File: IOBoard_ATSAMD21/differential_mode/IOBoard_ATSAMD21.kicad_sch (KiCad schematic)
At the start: 74 parts, among them IC1 AD8137YRZ-REEL, IC2 AD8137YRZ-REEL, J13 Eurorack_Mono_Jack, J3 Conn_PIC_ICSP_ICD, J5 Conn_01x05_Pin, J6 Conn_02x03_Odd_Even, SW1 EG_1218, SW2 EG_1218, SW3 EG_1218, SW4 EG_1218, U3 ATSAMD21G18A-A, U4 LM2904, U6 AP2112K-3.3

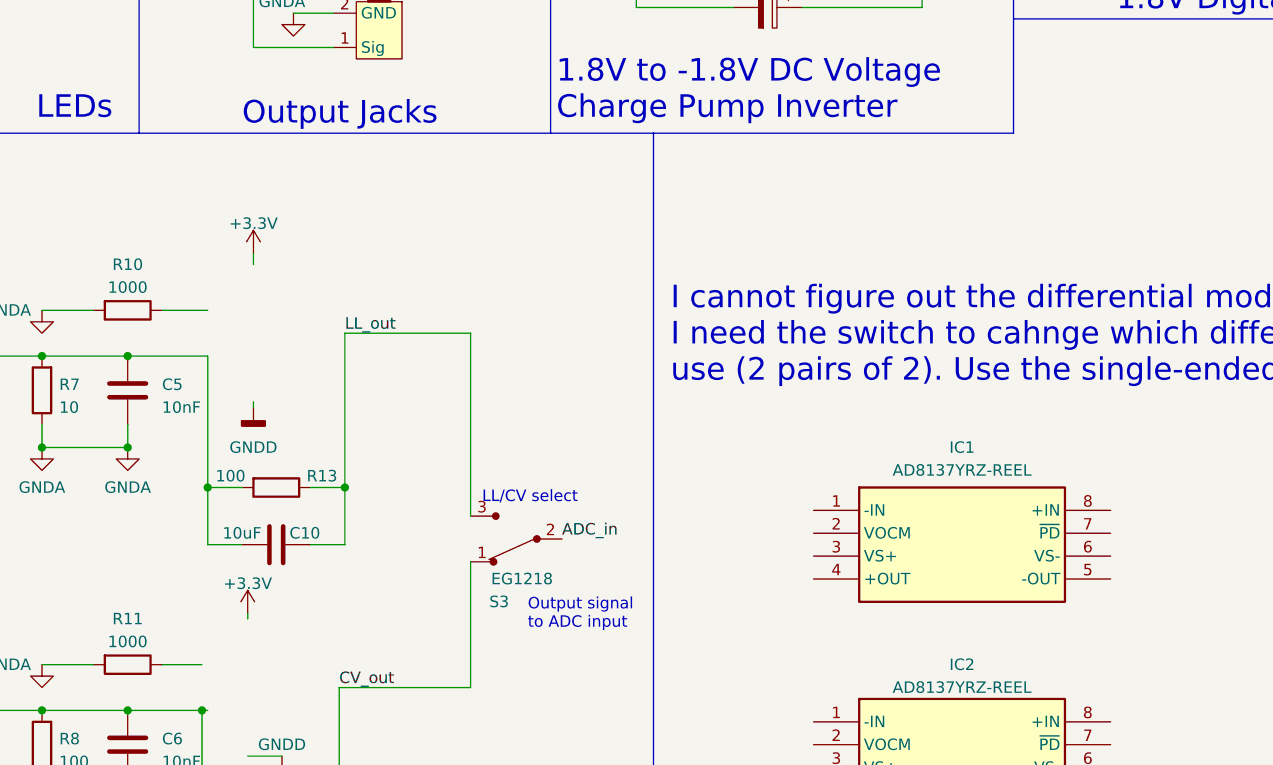
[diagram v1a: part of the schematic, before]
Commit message: plz work
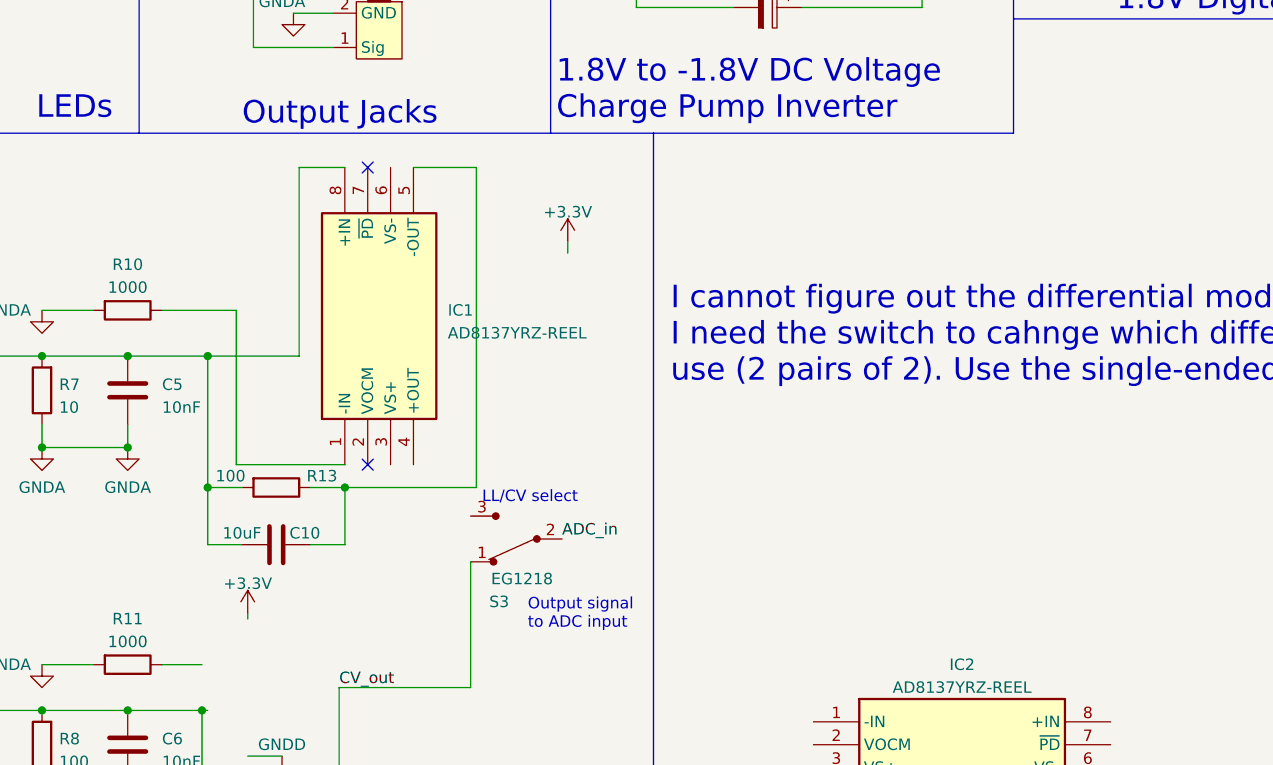
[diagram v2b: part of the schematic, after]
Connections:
- net LL_out: no longer C10.1, R13.1, S3.3
- net at C10.2, C5.2, R13.2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: now also IC1.8 (+IN)
- net at IC1.1 (-IN): now also R10.1
- net at IC1.5 (-OUT): now also C10.1, R13.1
- no-connect marks 7 -> 9
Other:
- moved on the sheet: IC1
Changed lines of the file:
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@@
   (junction (at 50.165 187.325) (diameter 0) (color 0 0 0 0)
   )
+  (junction (at 127 238.125) (diameter 0) (color 0 0 0 0)
+  )
   (junction (at 111.125 272.415) (diameter 0) (color 0 0 0 0)
   )
@@
   (junction (at 111.76 137.795) (diameter 0) (color 0 0 0 0)
   )
-  (junction (at 127 238.125) (diameter 0) (color 0 0 0 0)
-  )
   (junction (at 93.345 223.52) (diameter 0) (color 0 0 0 0)
   )
@@
   (junction (at 256.54 123.825) (diameter 0) (color 0 0 0 0)
   )
+  (junction (at 111.76 223.52) (diameter 0) (color 0 0 0 0)
+  )
   (junction (at 102.87 280.67) (diameter 0) (color 0 0 0 0)
   )
@@
   (no_connect (at 187.325 172.085))
   (no_connect (at 125.73 171.45))
+  (no_connect (at 129.54 202.565))
+  (no_connect (at 129.54 235.585))
   (no_connect (at 235.585 147.955))
   (no_connect (at 220.345 150.495))
@@
     (stroke (width 0) (type default))
   )
+  (wire (pts (xy 114.935 235.585) (xy 114.935 218.44))
+    (stroke (width 0) (type default))
+  )
   (wire (pts (xy 126.365 281.305) (xy 126.365 276.225))
     (stroke (width 0) (type default))
@@
     (stroke (width 0) (type default))
   )
+  (wire (pts (xy 121.92 202.565) (xy 121.92 223.52))
+    (stroke (width 0) (type default))
+  )
   (wire (pts (xy 114.3 64.135) (xy 121.92 64.135))
     (stroke (width 0) (type default))
@@
     (stroke (width 0) (type default))
   )
-  (wire (pts (xy 106.68 218.44) (xy 111.76 218.44))
+  (wire (pts (xy 106.68 218.44) (xy 114.935 218.44))
     (stroke (width 0) (type default))
   )
@@
     (stroke (width 0) (type default))
   )
-  (wire (pts (xy 140.97 241.3) (xy 140.97 220.98))
-    (stroke (width 0) (type default))
-  )
   (wire (pts (xy 137.16 20.955) (xy 137.16 26.035))
     (stroke (width 0) (type default))
@@
     (stroke (width 0) (type default))
   )
-  (wire (pts (xy 140.97 220.98) (xy 127 220.98))
-    (stroke (width 0) (type default))
-  )
   (polyline (pts (xy 201.295 198.755) (xy 201.295 159.385))
     (stroke (width 0) (type default))
@@
     (stroke (width 0) (type default))
   )
+  (wire (pts (xy 121.92 223.52) (xy 111.76 223.52))
+    (stroke (width 0) (type default))
+  )
   (wire (pts (xy 137.16 31.115) (xy 140.97 31.115))
     (stroke (width 0) (type default))
@@
     (stroke (width 0) (type default))
   )
-  (wire (pts (xy 116.84 229.235) (xy 116.84 228.6))
-    (stroke (width 0) (type default))
-  )
   (wire (pts (xy 266.7 34.925) (xy 271.78 34.925))
     (stroke (width 0) (type default))
@@
     (stroke (width 0) (type default))
   )
+  (wire (pts (xy 141.605 202.565) (xy 141.605 238.125))
+    (stroke (width 0) (type default))
+  )
   (wire (pts (xy 40.64 36.195) (xy 40.64 40.005))
     (stroke (width 0) (type default))
@@
     (stroke (width 0) (type default))
   )
-  (wire (pts (xy 116.84 212.09) (xy 116.84 213.36))
+  (wire (pts (xy 151.765 210.82) (xy 151.765 212.09))
     (stroke (width 0) (type default))
   )
@@
     (stroke (width 0) (type default))
   )
-  (wire (pts (xy 127 220.98) (xy 127 238.125))
-    (stroke (width 0) (type default))
-  )
   (wire (pts (xy 39.37 95.885) (xy 41.91 95.885))
     (stroke (width 0) (type default))
@@
     (stroke (width 0) (type default))
   )
+  (wire (pts (xy 134.62 202.565) (xy 141.605 202.565))
+    (stroke (width 0) (type default))
+  )
   (wire (pts (xy 114.3 64.135) (xy 114.3 69.215))
     (stroke (width 0) (type default))
@@
     (stroke (width 0) (type default))
   )
+  (wire (pts (xy 127 202.565) (xy 121.92 202.565))
+    (stroke (width 0) (type default))
+  )
   (polyline (pts (xy 215.9 104.775) (xy 215.9 127.635))
     (stroke (width 0) (type default))
@@
     (stroke (width 0) (type default))
   )
+  (wire (pts (xy 141.605 238.125) (xy 127 238.125))
+    (stroke (width 0) (type default))
+  )
   (wire (pts (xy 223.52 64.135) (xy 226.06 64.135))
     (stroke (width 0) (type default))
@@
     (stroke (width 0) (type default))
   )
+  (wire (pts (xy 127 235.585) (xy 114.935 235.585))
+    (stroke (width 0) (type default))
+  )
   (wire (pts (xy 241.3 64.135) (xy 241.3 53.975))
     (stroke (width 0) (type default))
@@
     (effects (font (size 1.27 1.27)) (justify left bottom))
   )
-  (label "LL_out" (at 127 220.98 0) (fields_autoplaced)
-    (effects (font (size 1.27 1.27)) (justify left bottom))
-  )
   (label "LED3" (at 72.39 164.465 90) (fields_autoplaced)
     (effects (font (size 1.27 1.27)) (justify left bottom))
@@
     )
   )
-  (symbol (lib_id "AD8137YRZ-REEL:AD8137YRZ-REEL") (at 179.07 240.665 0) (unit 1)
-    (in_bom yes) (on_board yes) (dnp no) (fields_autoplaced)
-    (property "Reference" "IC1" (at 195.58 233.68 0)
-      (effects (font (size 1.27 1.27)))
+  (symbol (lib_id "AD8137YRZ-REEL:AD8137YRZ-REEL") (at 127 235.585 90) (unit 1)
+    (in_bom yes) (on_board yes) (dnp no)
+    (property "Reference" "IC1" (at 138.43 218.44 90)
+      (effects (font (size 1.27 1.27)) (justify right))
     )
-    (property "Value" "AD8137YRZ-REEL" (at 195.58 236.22 0)
-      (effects (font (size 1.27 1.27)))
+    (property "Value" "AD8137YRZ-REEL" (at 138.43 220.98 90)
+      (effects (font (size 1.27 1.27)) (justify right))
     )
-    (property "Footprint" "SOIC127P600X175-8N" (at 208.28 335.585 0)
+    (property "Footprint" "SOIC127P600X175-8N" (at 221.92 206.375 0)
       (effects (font (size 1.27 1.27)) (justify left top) hide)
     )
-    (property "Datasheet" "https://www.arrow.com/en/products/ad8137yrz-reel/analog-devices" (at 208.28 435.585 0)
+    (property "Datasheet" "https://www.arrow.com/en/products/ad8137yrz-reel/analog-devices" (at 321.92 206.375 0)
       (effects (font (size 1.27 1.27)) (justify left top) hide)
     )
-    (property "Height" "1.75" (at 208.28 635.585 0)
+    (property "Height" "1.75" (at 521.92 206.375 0)
       (effects (font (size 1.27 1.27)) (justify left top) hide)
     )
-    (property "Manufacturer_Name" "Analog Devices" (at 208.28 735.585 0)
+    (property "Manufacturer_Name" "Analog Devices" (at 621.92 206.375 0)
       (effects (font (size 1.27 1.27)) (justify left top) hide)
     )
-    (property "Manufacturer_Part_Number" "AD8137YRZ-REEL" (at 208.28 835.585 0)
+    (property "Manufacturer_Part_Number" "AD8137YRZ-REEL" (at 721.92 206.375 0)
       (effects (font (size 1.27 1.27)) (justify left top) hide)
     )
-    (property "Mouser Part Number" "584-AD8137YRZ-R" (at 208.28 935.585 0)
+    (property "Mouser Part Number" "584-AD8137YRZ-R" (at 821.92 206.375 0)
       (effects (font (size 1.27 1.27)) (justify left top) hide)
     )
-    (property "Mouser Price/Stock" "https://www.mouser.co.uk/ProductDetail/Analog-Devices/AD8137YRZ-REEL?qs=%2FtpEQrCGXCwvx9BEhEk72g%3D%3D" (at 208.28 1035.585 0)
+    (property "Mouser Price/Stock" "https://www.mouser.co.uk/ProductDetail/Analog-Devices/AD8137YRZ-REEL?qs=%2FtpEQrCGXCwvx9BEhEk72g%3D%3D" (at 921.92 206.375 0)
       (effects (font (size 1.27 1.27)) (justify left top) hide)
     )
-    (property "Arrow Part Number" "AD8137YRZ-REEL" (at 208.28 1135.585 0)
+    (property "Arrow Part Number" "AD8137YRZ-REEL" (at 1021.92 206.375 0)
       (effects (font (size 1.27 1.27)) (justify left top) hide)
     )
-    (property "Arrow Price/Stock" "https://www.arrow.com/en/products/ad8137yrz-reel/analog-devices?region=nac" (at 208.28 1235.585 0)
+    (property "Arrow Price/Stock" "https://www.arrow.com/en/products/ad8137yrz-reel/analog-devices?region=nac" (at 1121.92 206.375 0)
       (effects (font (size 1.27 1.27)) (justify left top) hide)
     )
@@
     )
   )
-  (symbol (lib_id "power:+3.3V") (at 116.84 212.09 0) (unit 1)
+  (symbol (lib_id "power:+3.3V") (at 151.765 210.82 0) (unit 1)
     (in_bom yes) (on_board yes) (dnp no) (fields_autoplaced)
-    (property "Reference" "#PWR017" (at 116.84 215.9 0)
+    (property "Reference" "#PWR017" (at 151.765 214.63 0)
       (effects (font (size 1.27 1.27)) hide)
     )
-    (property "Value" "+3.3V" (at 116.84 208.7984 0)
+    (property "Value" "+3.3V" (at 151.765 207.5284 0)
       (effects (font (size 1.27 1.27)))
     )
-    (property "Footprint" "" (at 116.84 212.09 0)
+    (property "Footprint" "" (at 151.765 210.82 0)
       (effects (font (size 1.27 1.27)) hide)
     )
-    (property "Datasheet" "" (at 116.84 212.09 0)
+    (property "Datasheet" "" (at 151.765 210.82 0)
       (effects (font (size 1.27 1.27)) hide)
     )
@@
         )
       )
-    )
-  )
-  (symbol (lib_id "power:GNDD") (at 116.84 229.235 0) (unit 1)
-    (in_bom yes) (on_board yes) (dnp no) (fields_autoplaced)
-    (property "Reference" "#PWR018" (at 116.84 235.585 0)
-      (effects (font (size 1.27 1.27)) hide)
-    )
-    (property "Value" "GNDD" (at 116.84 233.68 0)
-      (effects (font (size 1.27 1.27)))
-    )
-    (property "Footprint" "" (at 116.84 229.235 0)
-      (effects (font (size 1.27 1.27)) hide)
-    )
-    (property "Datasheet" "" (at 116.84 229.235 0)
-      (effects (font (size 1.27 1.27)) hide)
-    )
-    (pin "1")
-    (instances
-      (project "IOBoard_ATSAMD21"
-        (path "/769f5a9c-d123-4372-b12b-6b5ae0bc94f0"
-          (reference "#PWR018") (unit 1)
-        )
-      )
